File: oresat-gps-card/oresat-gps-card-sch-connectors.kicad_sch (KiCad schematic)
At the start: 34 parts, among them J1 J-SAMTEC-TFM-120-01-L-D-RA, J3 J-TE-Debug-2-1734592-0

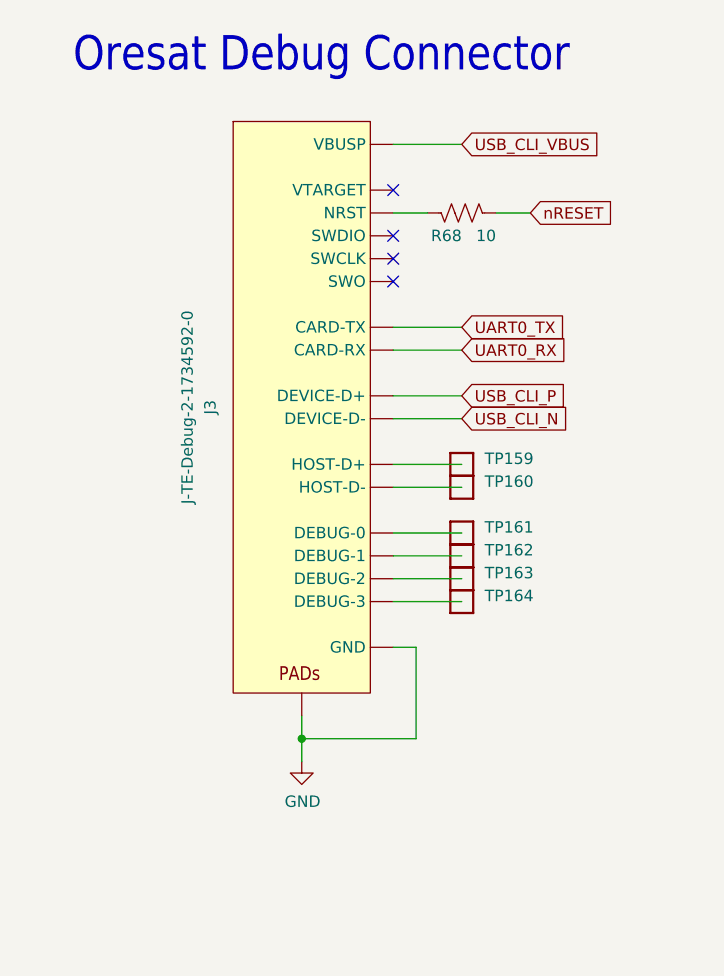
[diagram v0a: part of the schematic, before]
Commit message: Routine Push
Andrew should look at the MAX2769 change.
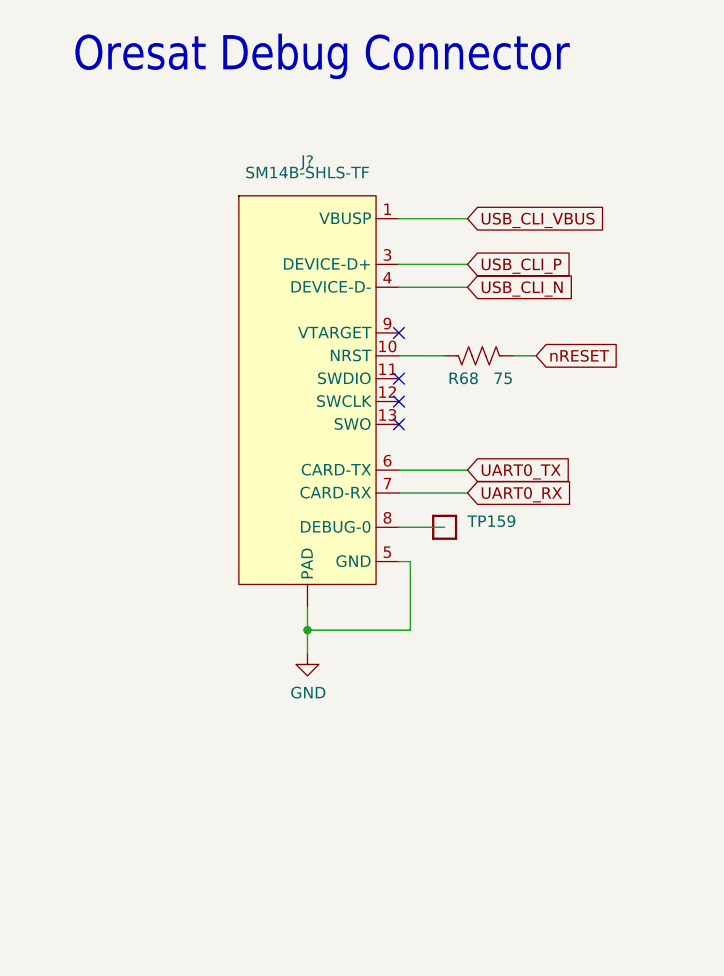
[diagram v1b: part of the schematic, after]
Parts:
- removed J3: J-TE-Debug-2-1734592-0, oresat-connectors:J-TE-2-1734592-0, symbol oresat-connectors:J-TE-2-1734592-0
- removed TP160, TP161, TP162, TP163, TP164: 0.03x0.04, oresat-misc:TestPoint_Pad_D1.0mm, symbol oresat-misc:Test-Point-1mm-round
- added J?: SM14B-SHLS-TF, oresat-connectors:J-JST-SM14BSHLSTF, symbol oresat-connectors:ORESAT-DEBUG-CONNECTOR-3
- R68: value 10 -> 75
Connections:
- net GND: now also J?.14 (GND), J?.15 (PAD), J?.16 (PAD), J?.5 (GND)
- net UART0_RX: now also J?.7 (CARD-RX)
- net UART0_TX: now also J?.6 (CARD-TX)
- net USB_CLI_N: now also J?.4 (DEVICE-D-)
- net USB_CLI_P: now also J?.3 (DEVICE-D+)
- net USB_CLI_VBUS: now also J?.1 (VBUSP), J?.2 (VBUSP)
- net at TP159.1: now also J?.8 (DEBUG-0)
- net at R68.1: now also J?.10 (NRST)
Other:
- moved on the sheet: R68, TP159

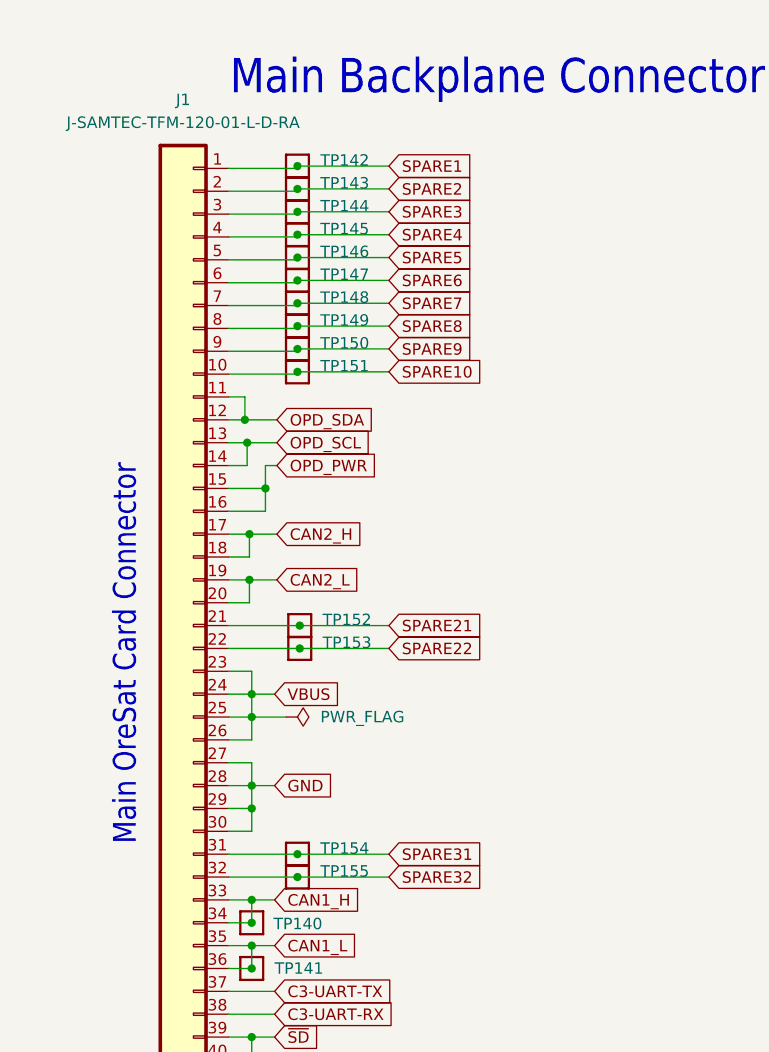
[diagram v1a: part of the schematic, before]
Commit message: Routine Push
Various small changes made
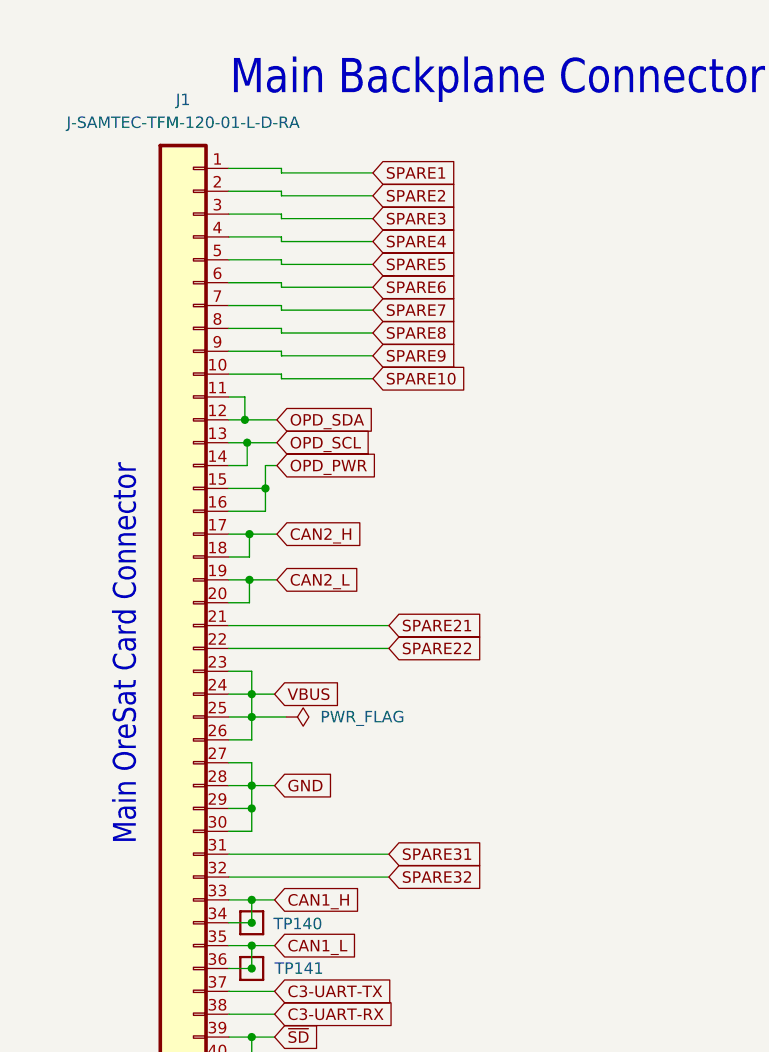
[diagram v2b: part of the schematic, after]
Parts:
- removed TP142, TP143, TP144, TP145, TP146, TP147, TP148, TP149, TP150, TP151, TP152, TP153, TP154, TP155: 0.03x0.04, oresat-misc:TestPoint_Pad_D1.0mm, symbol oresat-misc:Test-Point-1mm-round

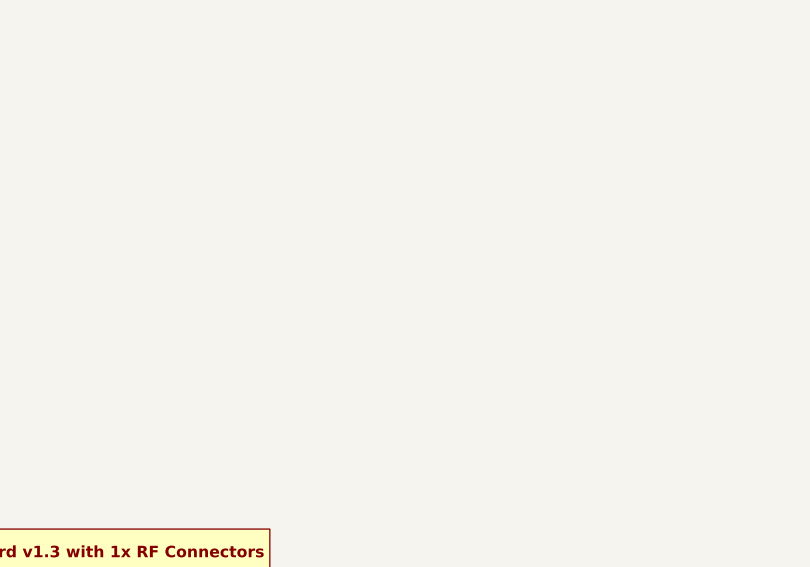
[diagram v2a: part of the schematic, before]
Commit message: Routine Push
First attempt to clean up schematic
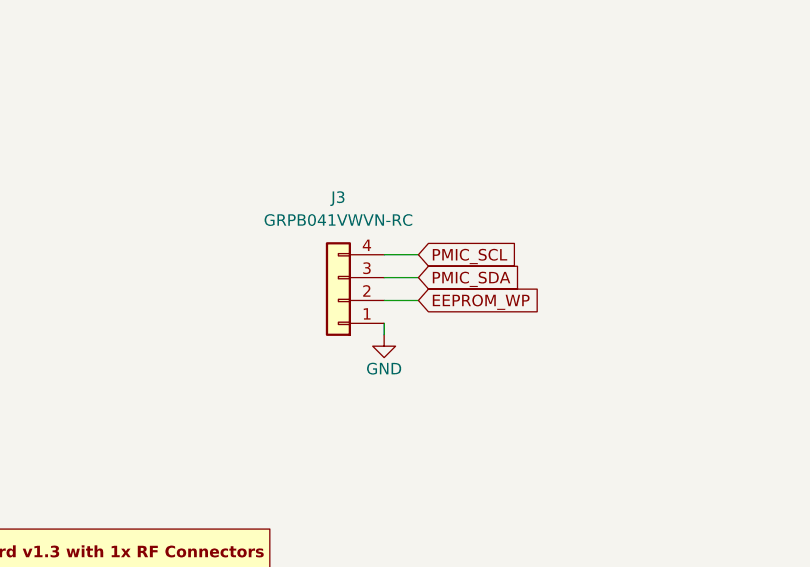
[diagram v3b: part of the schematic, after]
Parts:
- added J3: GRPB041VWVN-RC, Connector_PinHeader_1.27mm:PinHeader_1x04_P1.27mm_Vertical, symbol Connector_Generic:Conn_01x04
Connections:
- net GND: now also J3.1 (Pin_1)
- new net EEPROM_WP: J3.2 (Pin_2)
- new net PMIC_SCL: J3.4 (Pin_4)
- new net PMIC_SDA: J3.3 (Pin_3)
